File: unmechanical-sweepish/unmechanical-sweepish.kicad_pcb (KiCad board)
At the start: 4 copper layers, 252.8 x 128.9 mm, 168 parts, among them J1 HytePro M, J2 USB_C_Receptacle_USB2.0, J3 M, J4 HytePro F, J5 USB_C_Receptacle_USB2.0, J6 M, Q1 AO3400A, Q2 AO3400A, SW1 B/R, SW2 B/R, U1 XC6206PxxxMR, U10 74HC4051, U2 SRV05-4, U3 STM32G431CBUx, U4 OPA340NA, U5 74HC4051, U6 XC6206PxxxMR, U7 SRV05-4, U8 STM32G431CBUx, U9 OPA340NA

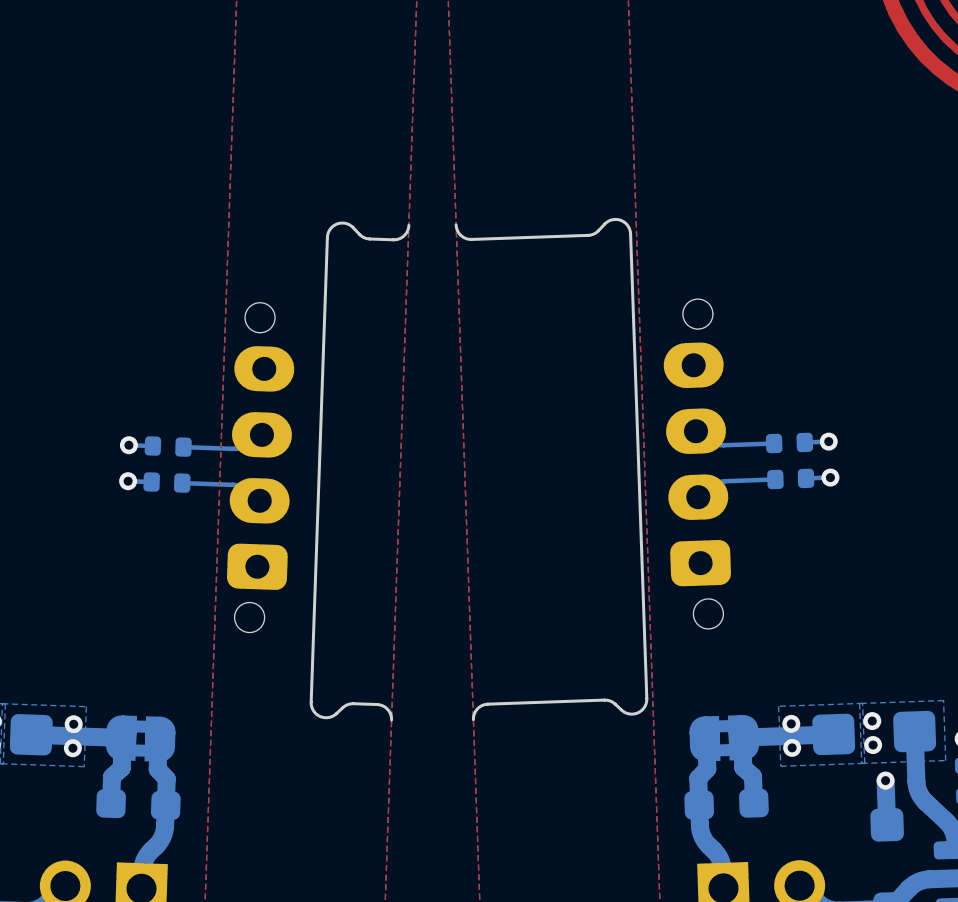
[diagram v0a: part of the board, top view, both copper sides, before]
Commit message: Fix up for order
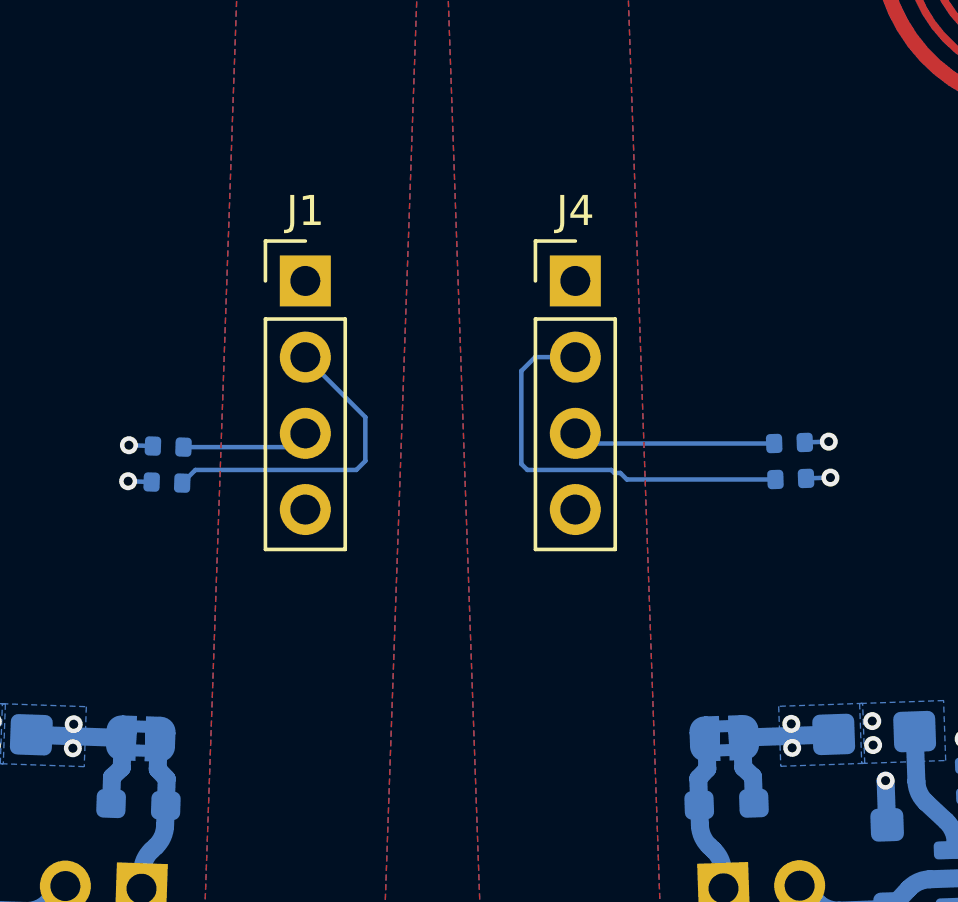
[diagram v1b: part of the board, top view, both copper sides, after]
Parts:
- J1: footprint PCM_marbastlib-xp-various:CON_HytePro_M411P_Plug_1x04-P2.20mm_Horizontal_FlushMount -> Connector_PinHeader_2.54mm:PinHeader_1x04_P2.54mm_Vertical; moved to F.Cu
- J4: footprint PCM_marbastlib-xp-various:CON_HytePro_M411P_Receptacle_1x04-P2.20mm_Horizontal_FlushMount -> Connector_PinHeader_2.54mm:PinHeader_1x04_P2.54mm_Vertical; moved to F.Cu
- L1, L2: value BLM15PX121SN1D -> BLM15PX121SN1D
- moved J4 10.3 mm to (158.0, 82.6), turned to 0 degrees
- moved J1 9.66 mm to (149.0, 82.6), turned to 0 degrees
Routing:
- net Net-(J4-Pin_2): track 2.75 -> 13.8 mm
- net Net-(J1-Pin_2): track 2.76 -> 10.7 mm
- net Net-(J4-Pin_3): track 2.75 -> 6.77 mm
- net Net-(J1-Pin_3): track 2.76 -> 4.25 mm
